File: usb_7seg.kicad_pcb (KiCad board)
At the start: 2 copper layers, 72 x 47 mm, 8 parts, among them IC1 MAX7219CNG, IC2 MAX7219CWG, U1 SeeeduinoXIAO, U2 7segment_led

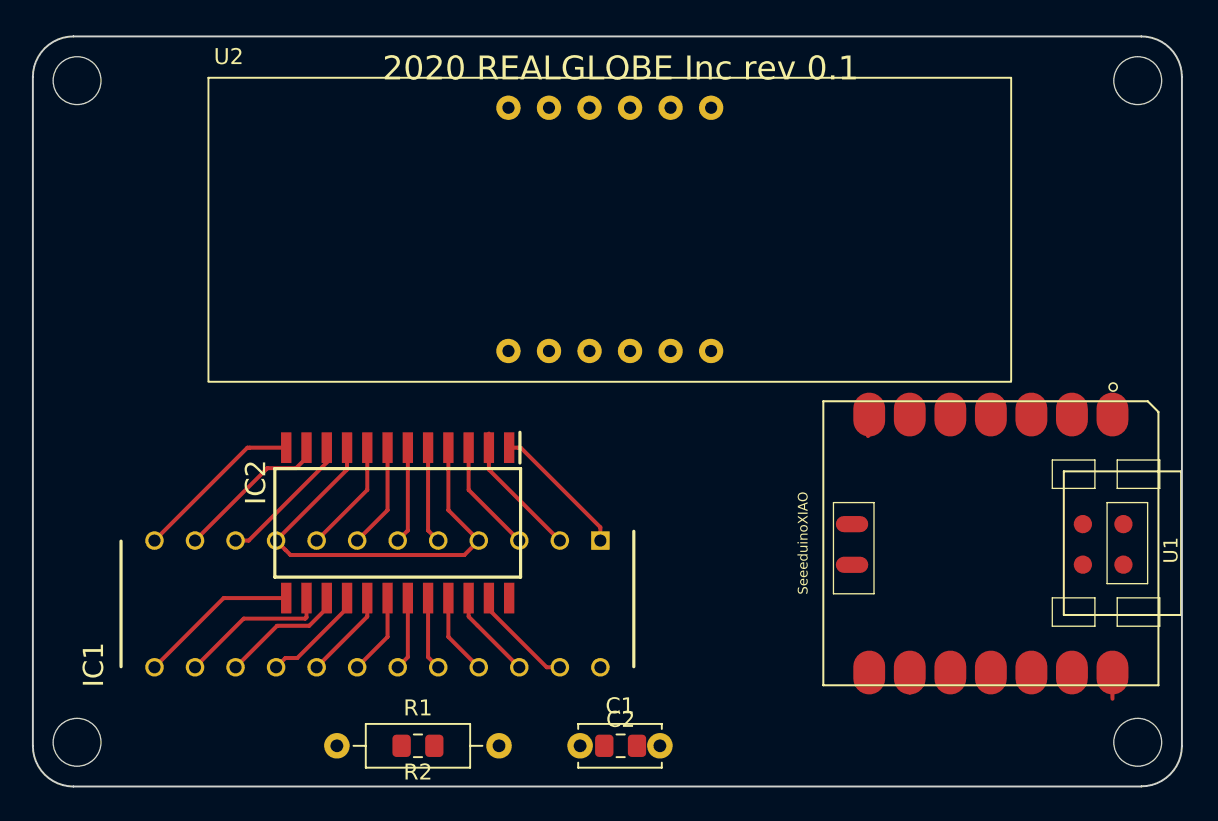
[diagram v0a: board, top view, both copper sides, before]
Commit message: とりあえず完成。DRCもok
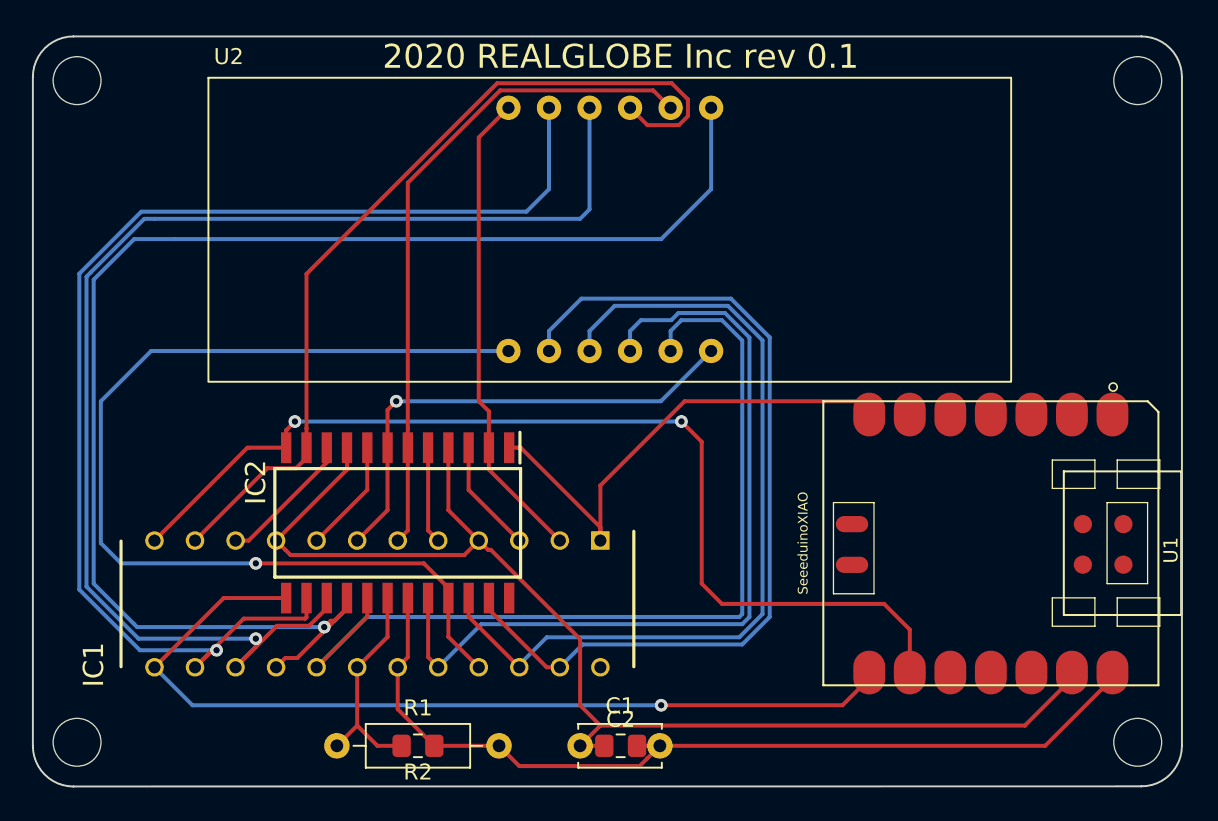
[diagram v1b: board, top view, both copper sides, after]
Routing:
- net Net-(IC1-Pad16): track 6.62 -> 89.3 mm, vias 0 -> 1
- net Net-(IC1-Pad15): track 7.89 -> 81.2 mm, vias 0 -> 1
- net Net-(IC1-Pad14): track 9.49 -> 78.0 mm, vias 0 -> 1
- net Net-(IC1-Pad21): track 5.76 -> 64.4 mm, vias 0 -> 1
- net Net-(IC1-Pad12): track 11.0 -> 64.4 mm, vias 0 -> 2
- net +5V: track 4.98 -> 57.6 mm
- net Net-(IC1-Pad17): track 5.65 -> 57.4 mm
- net GND: track 27.7 -> 77.0 mm
- net Net-(IC1-Pad23): track 7.46 -> 56.4 mm
- net Net-(IC1-Pad20): track 4.60 -> 52.8 mm
- net Net-(IC1-Pad22): track 6.29 -> 53.8 mm
- net Net-(IC1-Pad13): track 10.1 -> 56.9 mm, vias 0 -> 1
- net Net-(IC1-Pad11): track 10.4 -> 55.9 mm
- net Net-(IC1-Pad6): track 6.09 -> 42.0 mm
- net Net-(IC1-Pad7): track 6.61 -> 30.8 mm, vias 0 -> 1
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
